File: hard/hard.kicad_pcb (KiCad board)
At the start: 2 copper layers, 138.1 x 118.7 mm, 72 parts, among them J1 USB_C_Receptacle_USB2.0, J2 RJ45_LED_Shielded, SW1 SW_RST, SW10 KEY_Q, SW11 KEY_A, SW12 KEY_OPTION, SW13 KEY_2, SW14 KEY_Z, SW15 KEY_W, SW16 KEY_S, SW17 KEY_COMMAND, SW18 KEY_3, SW19 KEY_X, SW2 SW_BOOT0, SW20 KEY_E, SW21 KEY_D, SW22 KEY_4, SW23 KEY_C, SW24 KEY_R, SW25 KEY_F, SW26 KEY_5, SW27 KEY_SPACE, SW28 KEY_V, SW29 KEY_T, SW3 KEY_CAPSLOCK, SW30 KEY_G, SW31 KEY_6, SW32 KEY_B, SW4 KEY_LSHIFT, SW5 KEY_LFN, SW6 KEY_TAB, SW7 KEY_ESCAPE, SW8 KEY_CONTROL, SW9 KEY_1, U1 THVD1451D, U2 USBLC6-2SC6, U3 MIC5504-3.3YM5, U4 STLinkV3, U5 STM32L412RBTx, Y1 8MHz

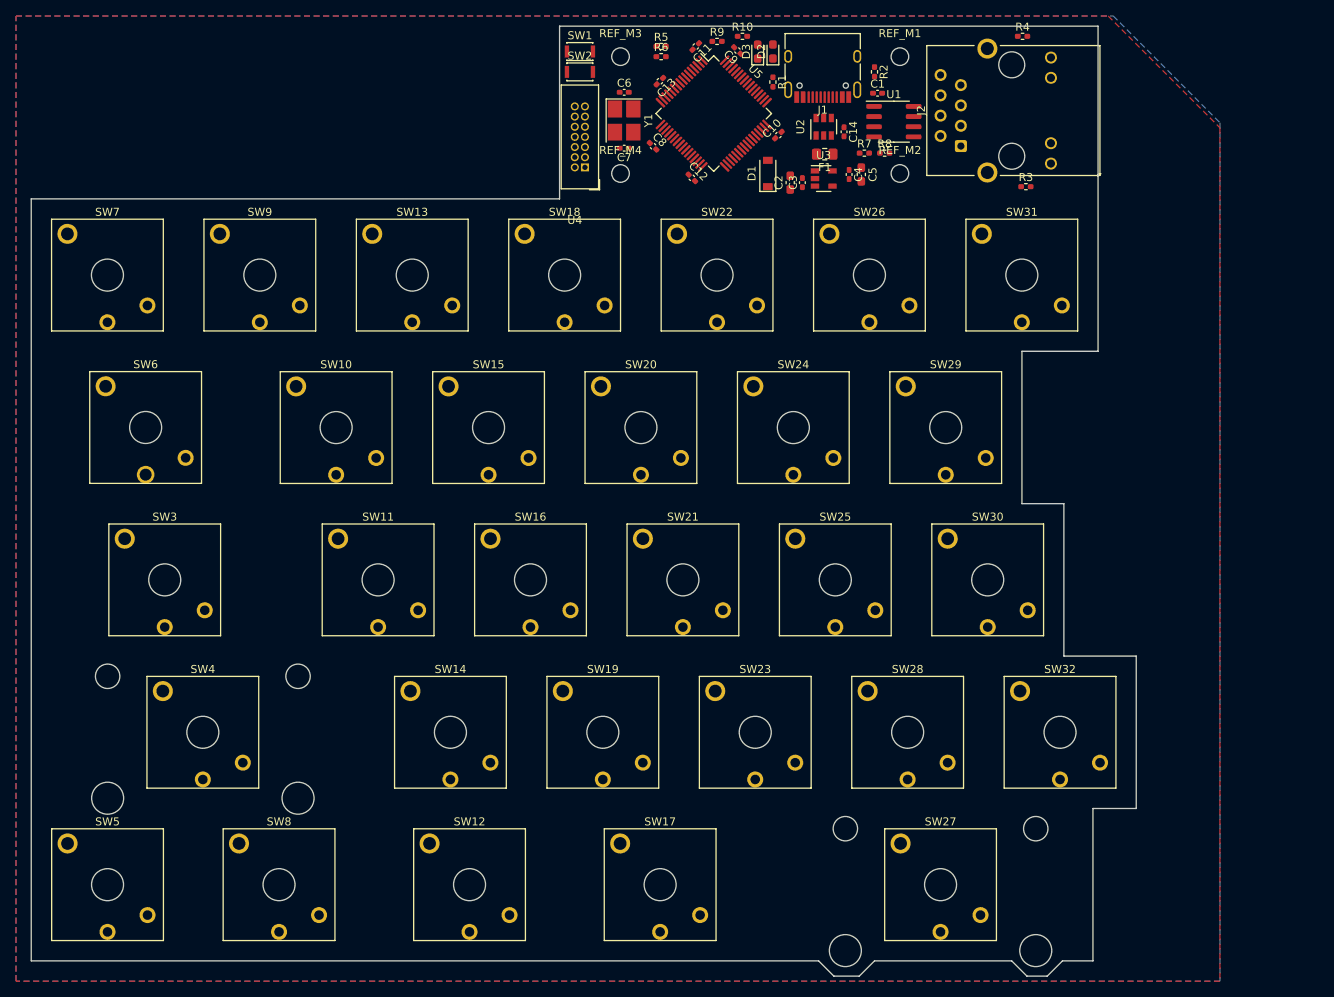
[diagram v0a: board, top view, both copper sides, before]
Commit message: hard: new shape
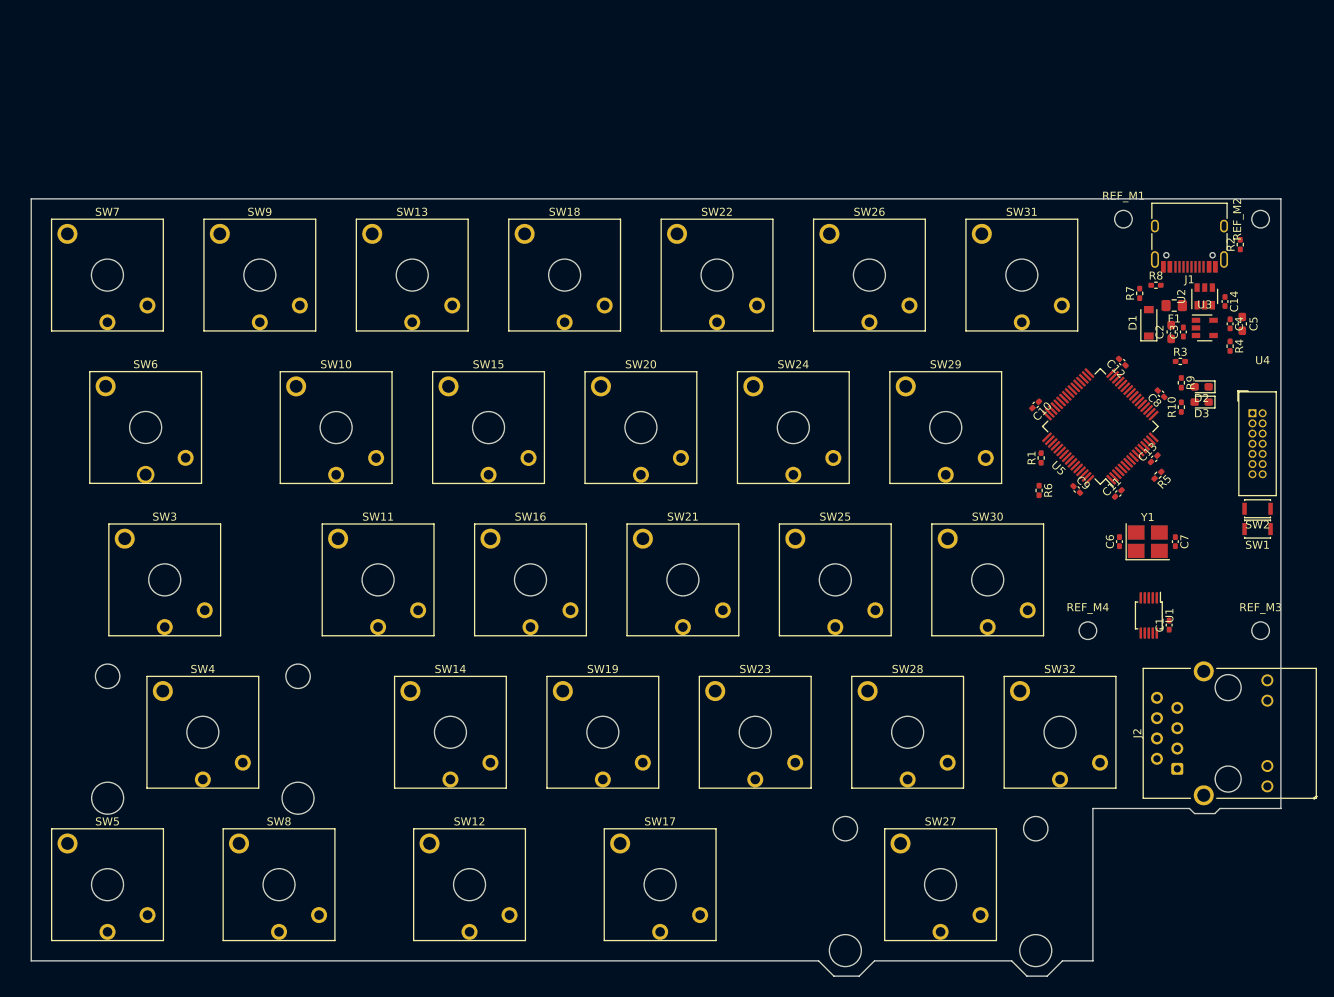
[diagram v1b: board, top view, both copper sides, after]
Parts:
- U1: value THVD1451D -> LTC2852xMS; footprint Package_SO:SOIC-8_3.9x4.9mm_P1.27mm -> Package_SO:MSOP-10_3x3mm_P0.5mm
- moved REF_M3 107.5 mm to (233.0, 120.0)
- moved SW1 103.6 mm to (232.7, 107.3), turned to 180 degrees
- moved SW2 100.8 mm to (232.7, 104.8), turned to 180 degrees
- moved U4 88.9 mm to (232.0, 92.8), turned to 0 degrees
- moved C7 84.6 mm to (222.4, 108.9), turned to 270 degrees
- moved Y1 84.0 mm to (218.9, 108.9), turned to 0 degrees
- moved C6 83.6 mm to (215.4, 108.9), turned to 90 degrees
- moved J2 82.4 mm to (222.6, 137.3)
- moved R5 82.0 mm to (220.2, 100.6), turned to 225 degrees
- moved REF_M4 81.7 mm to (211.5, 120.0)
- moved C13 77.8 mm to (219.7, 98.5), turned to 45 degrees
- moved C11 76.9 mm to (215.3, 102.9), turned to 45 degrees
- moved C1 75.8 mm to (221.6, 119.3), turned to 90 degrees
- moved R9 72.0 mm to (223.1, 89.0), turned to 270 degrees
- moved R6 71.9 mm to (205.4, 102.5), turned to 270 degrees
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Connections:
- C14 pad 1: /V_SHARED -> Net-(C14-Pad1)
- C2 pad 1: Net-(C2-Pad1) -> /V_SHARED
- C3 pad 1: Net-(C2-Pad1) -> /V_SHARED
- D1 pad 1: Net-(C2-Pad1) -> /V_SHARED
- D1 pad 2: /V_SHARED -> Net-(C14-Pad1)
- F1 pad 1: /V_SHARED -> Net-(C14-Pad1)
- J1 pad A8: (no net) -> Net-(J1-PadA8)
- J1 pad B8: (no net) -> Net-(J1-PadB8)
- R7 pad 1: Net-(C2-Pad1) -> Net-(C14-Pad1)
- U1 pad 1: +3V3 -> /RX
- U1 pad 2: /RX -> GND
- U1 pad 3: /TX -> +3V3
- U1 pad 4: GND -> /TX
- U1 pad 5: /ETH_TX- -> GND
- U1 pad 6: /ETH_TX+ -> /ETH_TX-
- U1 pad 7: /ETH_RX- -> /ETH_TX+
- U1 pad 8: /ETH_RX+ -> /ETH_RX-
- U2 pad 5: /V_SHARED -> Net-(C14-Pad1)
- U3 pad 1: Net-(C2-Pad1) -> /V_SHARED
- U3 pad 3: Net-(C2-Pad1) -> /V_SHARED
- U3 pad 4: (no net) -> Net-(U3-Pad4)
- U4 pad 1: (no net) -> Net-(U4-Pad1)
- U4 pad 2: (no net) -> Net-(U4-Pad2)
- U5 pad 14: (no net) -> Net-(U5-Pad14)
- U5 pad 15: (no net) -> Net-(U5-Pad15)
- U5 pad 30: (no net) -> Net-(U5-Pad30)
- U5 pad 4: (no net) -> Net-(U5-Pad4)
- U5 pad 61: (no net) -> Net-(U5-Pad61)
- U5 pad 62: (no net) -> Net-(U5-Pad62)
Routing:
- removed copper zone on B.Cu, net GND
- removed copper zone on F.Cu, net GND
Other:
- board size 138.1 x 118.7 mm -> 156.2 x 97.2 mm
